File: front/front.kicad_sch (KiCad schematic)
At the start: 0 parts

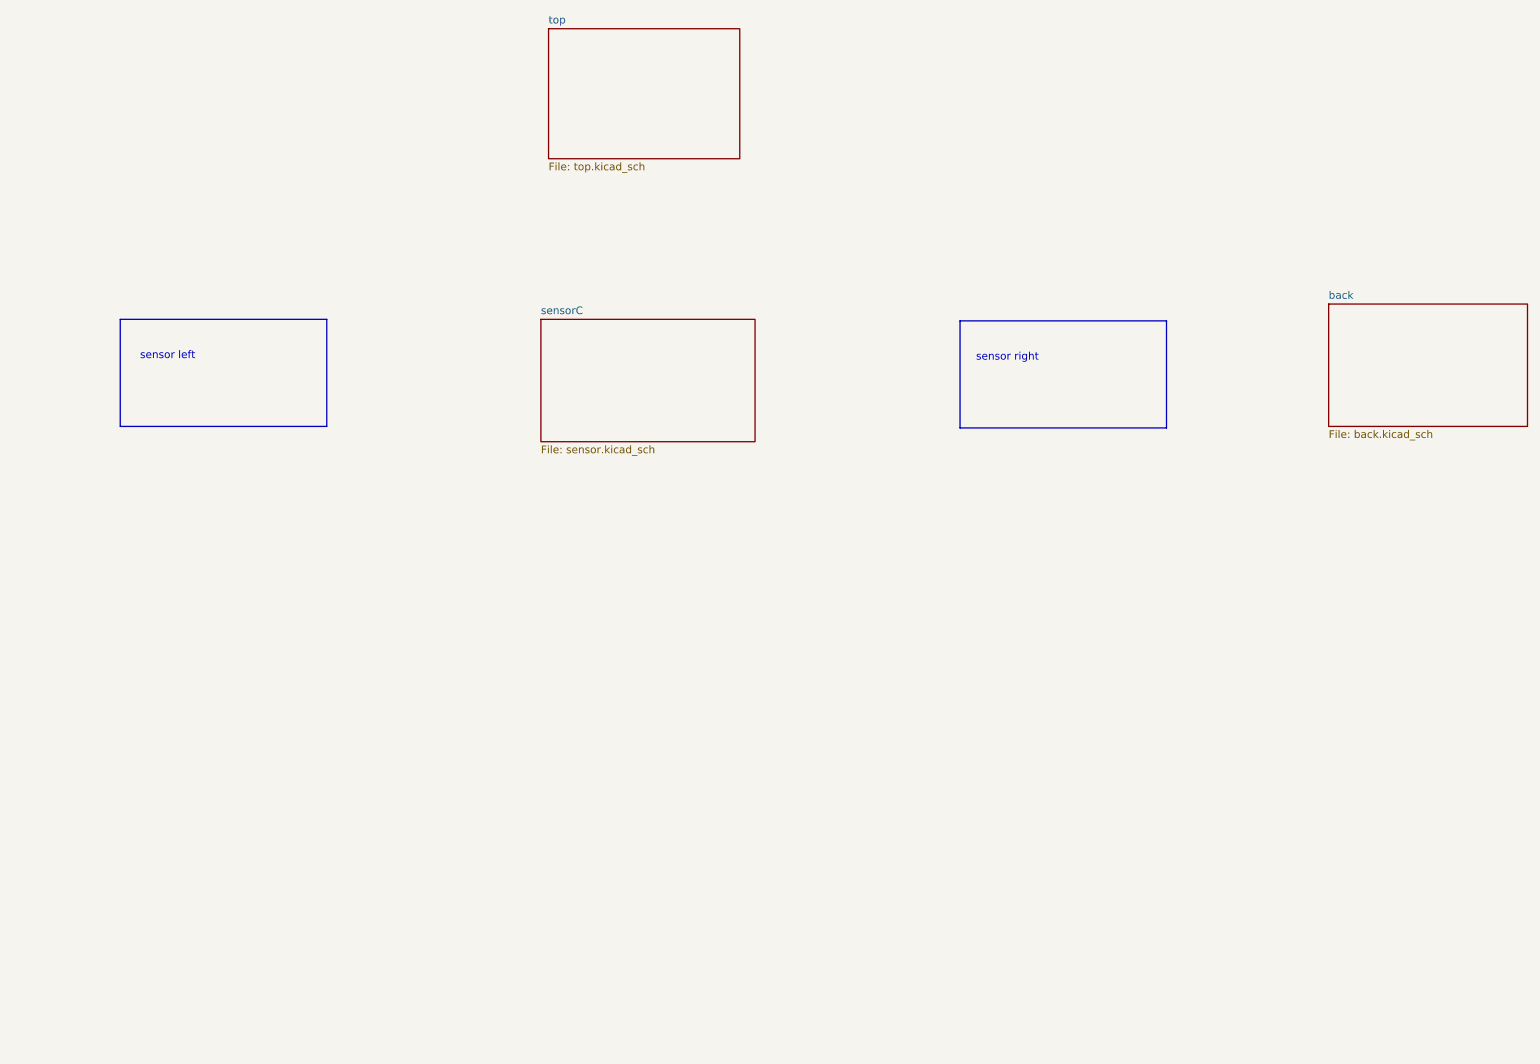
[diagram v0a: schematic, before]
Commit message: begin layout
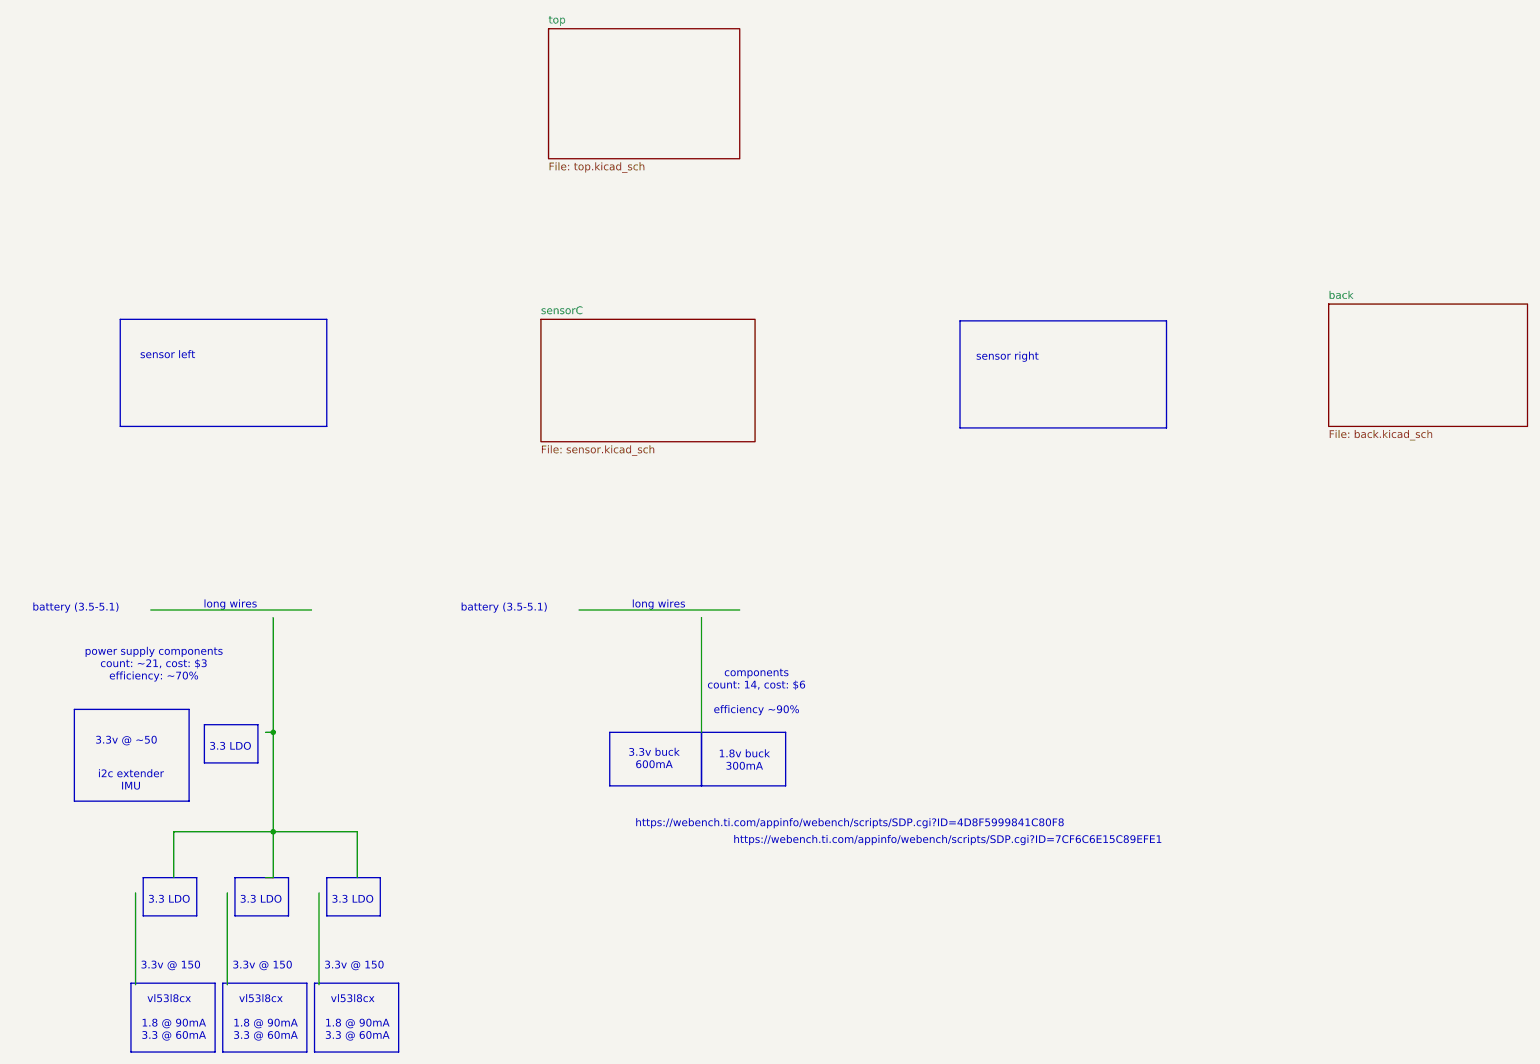
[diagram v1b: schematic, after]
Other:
- note added: "1.8 @ 90mA 3.3 @ 60mA"
- note added: "1.8v buck 300mA"
- note added: "3.3 LDO"
- note added: "3.3v @ 150"
- note added: "3.3v @ ~50"
- note added: "3.3v buck 600mA"
- note added: "battery (3.5-5.1)"
- note added: "components count: 14, cost: $6 efficiency ~90%"
- note added: "https://webench.ti.com/appinfo/webench/scripts/SDP.cgi?ID=4D8F5999841C80F8"
- note added: "https://webench.ti.com/appinfo/webench/scripts/SDP.cgi?ID=7CF6C6E15C89EFE1"
- note added: "i2c extender IMU"
- note added: "long wires"
- note added: "power supply components count: ~21, cost: $3 efficiency: ~70%"
- note added: "vl53l8cx"
